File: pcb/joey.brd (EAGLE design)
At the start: 42.3 x 49.3 mm, 62 parts, among them J1 AVR_SPI_PRG_6PTH, U1 ATMEGA168, U2 TMP102, X1 USB-MICROB, Y1 13.56M

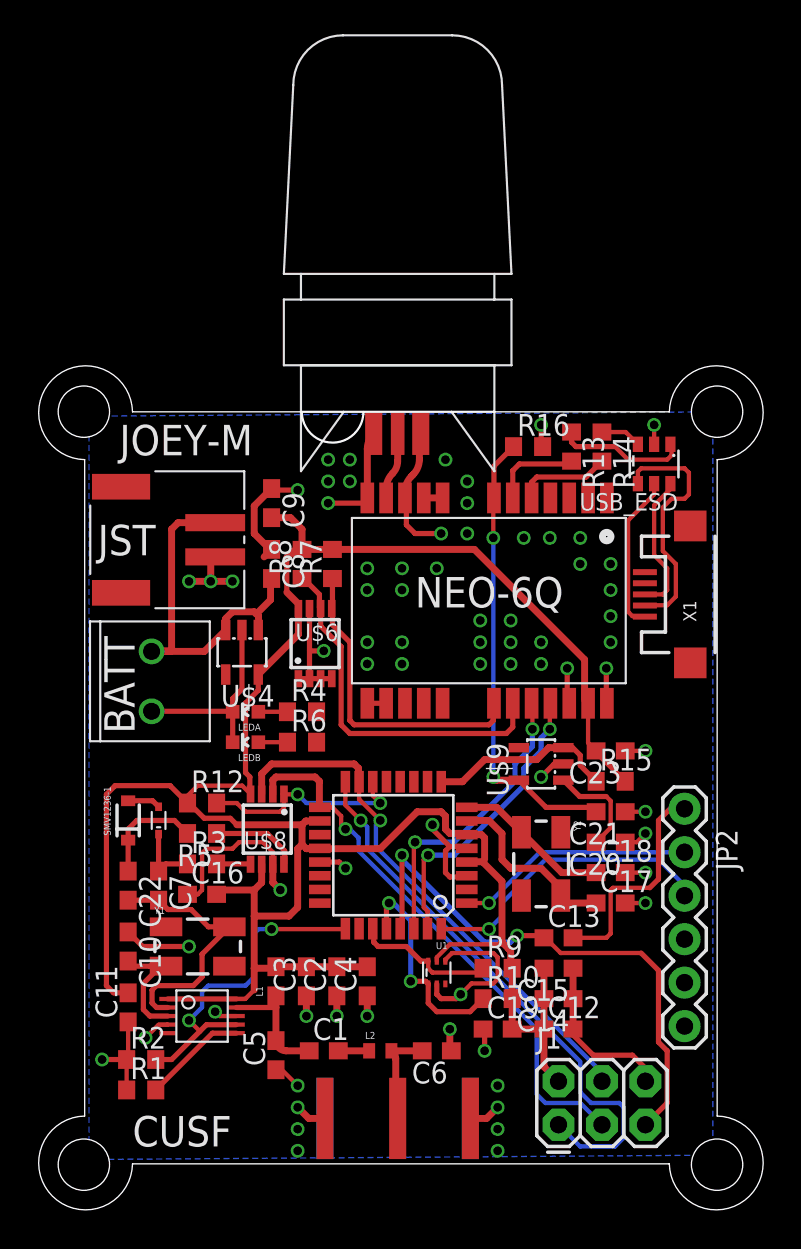
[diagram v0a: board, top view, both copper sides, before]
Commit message: Finished routing for v1.0
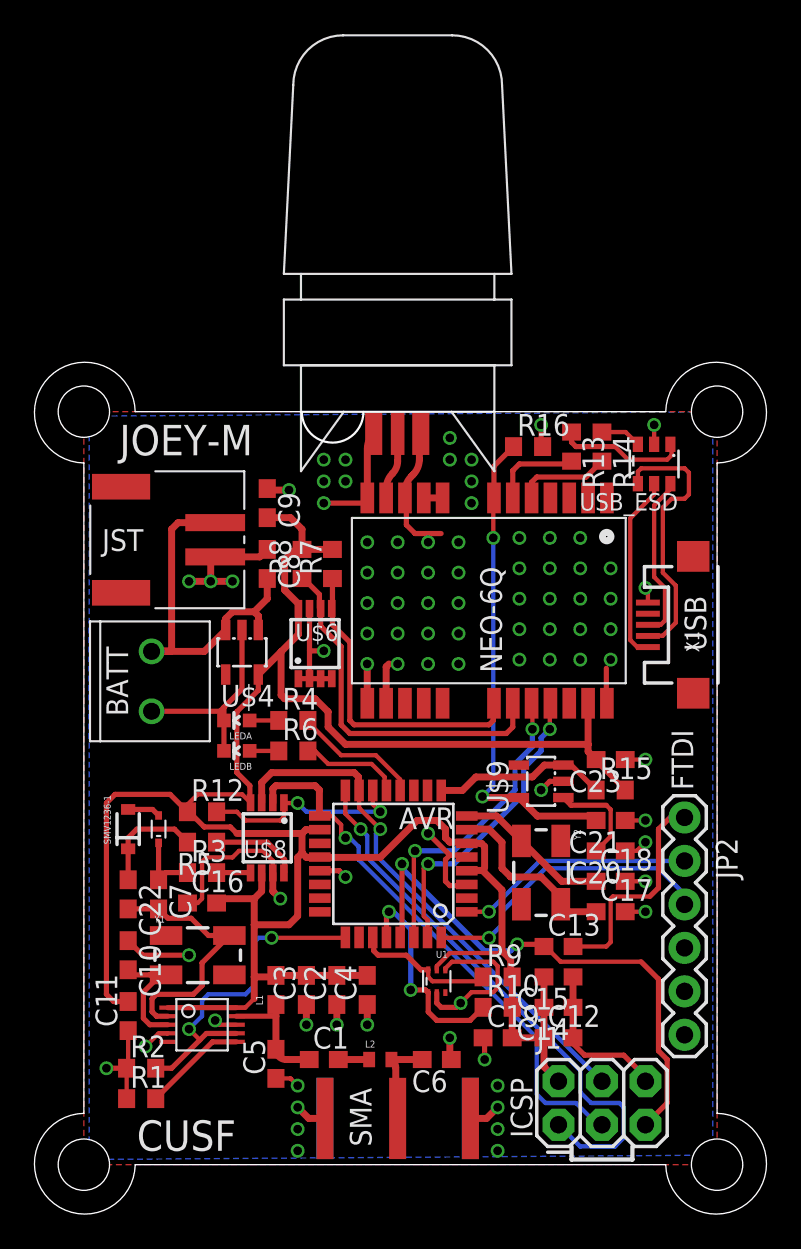
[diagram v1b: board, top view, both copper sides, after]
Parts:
- moved X1 1.79 mm to (38.6, 34.5)
- moved U$9 1.02 mm to (29.7, 25.4)
- moved LEDA 0.72 mm to (11.9, 29.0)
- moved LEDB 0.72 mm to (11.9, 27.2)
- moved R4 0.72 mm to (15.2, 29.0)
- moved R6 0.72 mm to (15.2, 27.2)
- moved C20 0.51 mm to (33.8, 21.3)
- moved R3 0.51 mm to (9.91, 20.1)
- moved U$8 0.51 mm to (13.7, 22.1)
- moved Y2 0.51 mm to (29.7, 20.1)
- moved C11 0.51 mm to (5.59, 11.7)
- moved C12 0.51 mm to (30.7, 10.4)
- moved C13 0.51 mm to (30.7, 15.7)
- moved C19 0.51 mm to (27.2, 10.4)
- moved R2 0.51 mm to (6.35, 8.64)
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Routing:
- net LEDA: track 0.00 -> 7.51 mm
- net LEDB: track 0.00 -> 5.95 mm
- net VCC: track 146.7 -> 150.0 mm
- net VBUS_3V3: track 26.9 -> 28.5 mm
- net N$16: track 9.32 -> 10.9 mm
- net N$18: track 14.5 -> 16.0 mm
- net N$19: track 8.33 -> 9.75 mm
- net GPS_USB_EN: track 11.0 -> 10.3 mm
- net SCK: track 32.4 -> 31.9 mm
- net MOSI: track 32.0 -> 31.5 mm
- net N$7: track 5.87 -> 5.36 mm
- net GPS_TX: track 17.3 -> 17.8 mm
- net GPS_RX: track 17.5 -> 18.0 mm
- net RESET: track 32.3 -> 31.8 mm
- net MISO: track 33.1 -> 32.5 mm
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- added copper zone on layer 1, net GND
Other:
- board size 42.3 x 49.3 mm -> 42.8 x 49.8 mm
- board text added: "AVR"
- board text added: "BLK"
- board text added: "FTDI"
- board text added: "GRN"
- board text added: "ICSP"
- board text added: "MAR '12"
- board text added: "SMA"
- board text added: "USB"
- board text added: "v1.0"
